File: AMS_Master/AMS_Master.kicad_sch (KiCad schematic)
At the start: 55 parts, among them IC1 LTM2884CY#PBF, IC2 LTC4411ES5#TRMPBF, IC3 ISO1042DWVR, J1 Conn_01x04_Pin, J2 Conn_01x04_Pin, J3 USB_B, J4 Conn_01x14_Pin, U1 LD1117S50TR_SOT223, U2 ADuM1250, U3 MCP2515-xSO, U4 ATmega328P-A, U5 FT232RL, Y1 Crystal, Y2 CSTCE16M0V53-R0

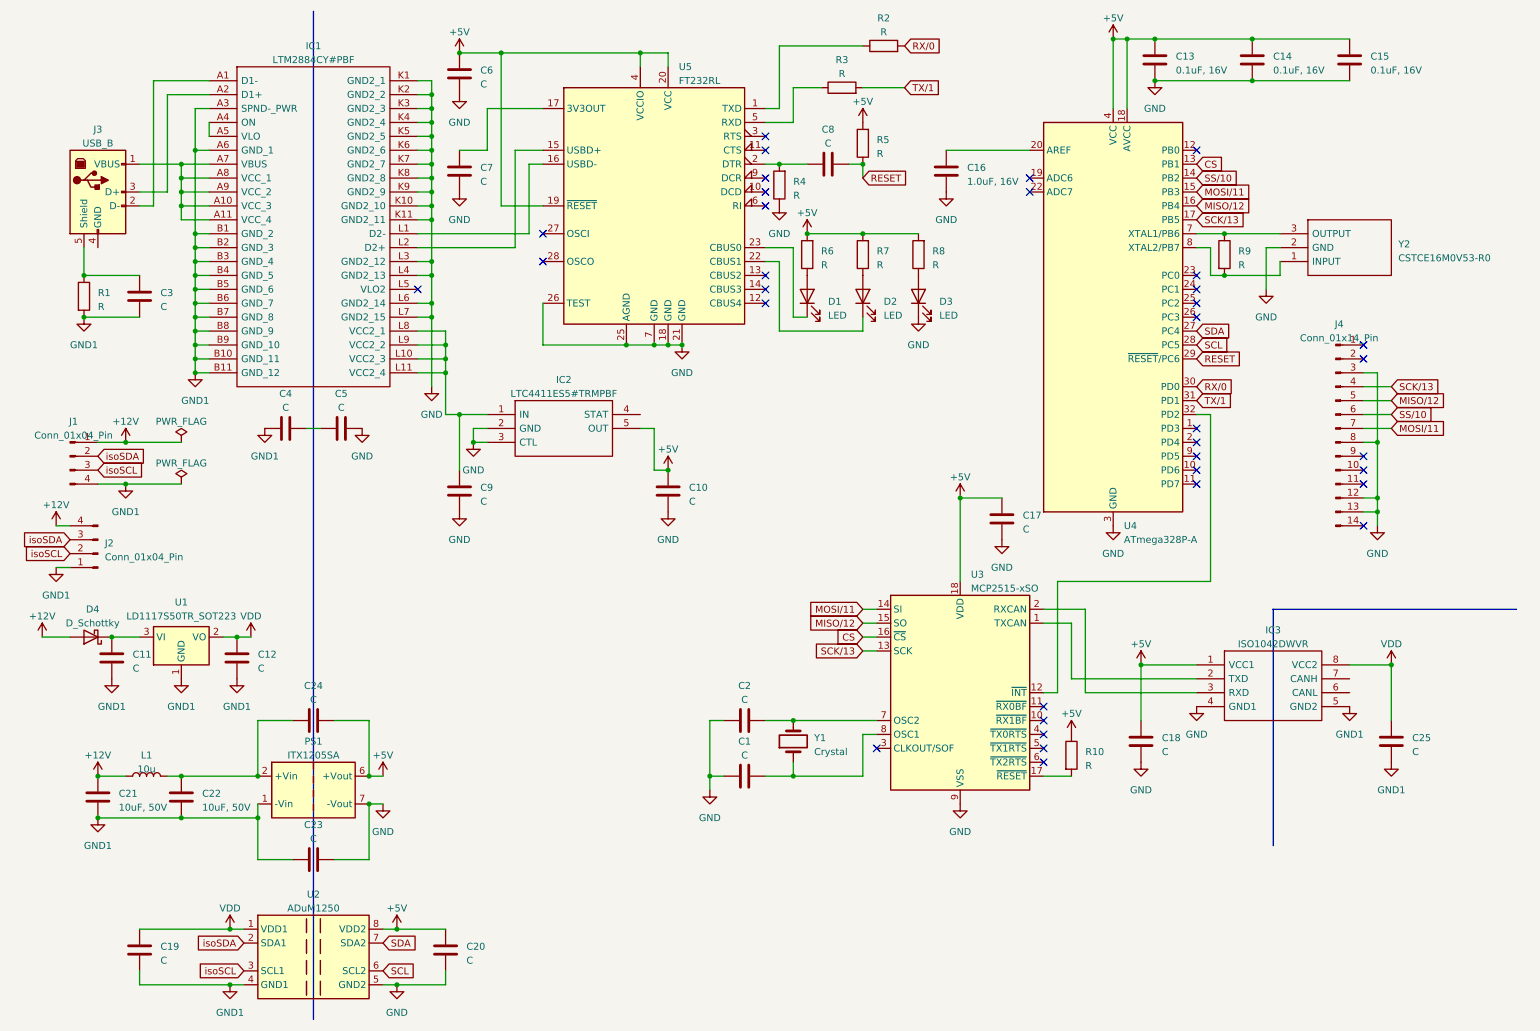
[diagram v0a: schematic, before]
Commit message: AMS_Master回路図更新
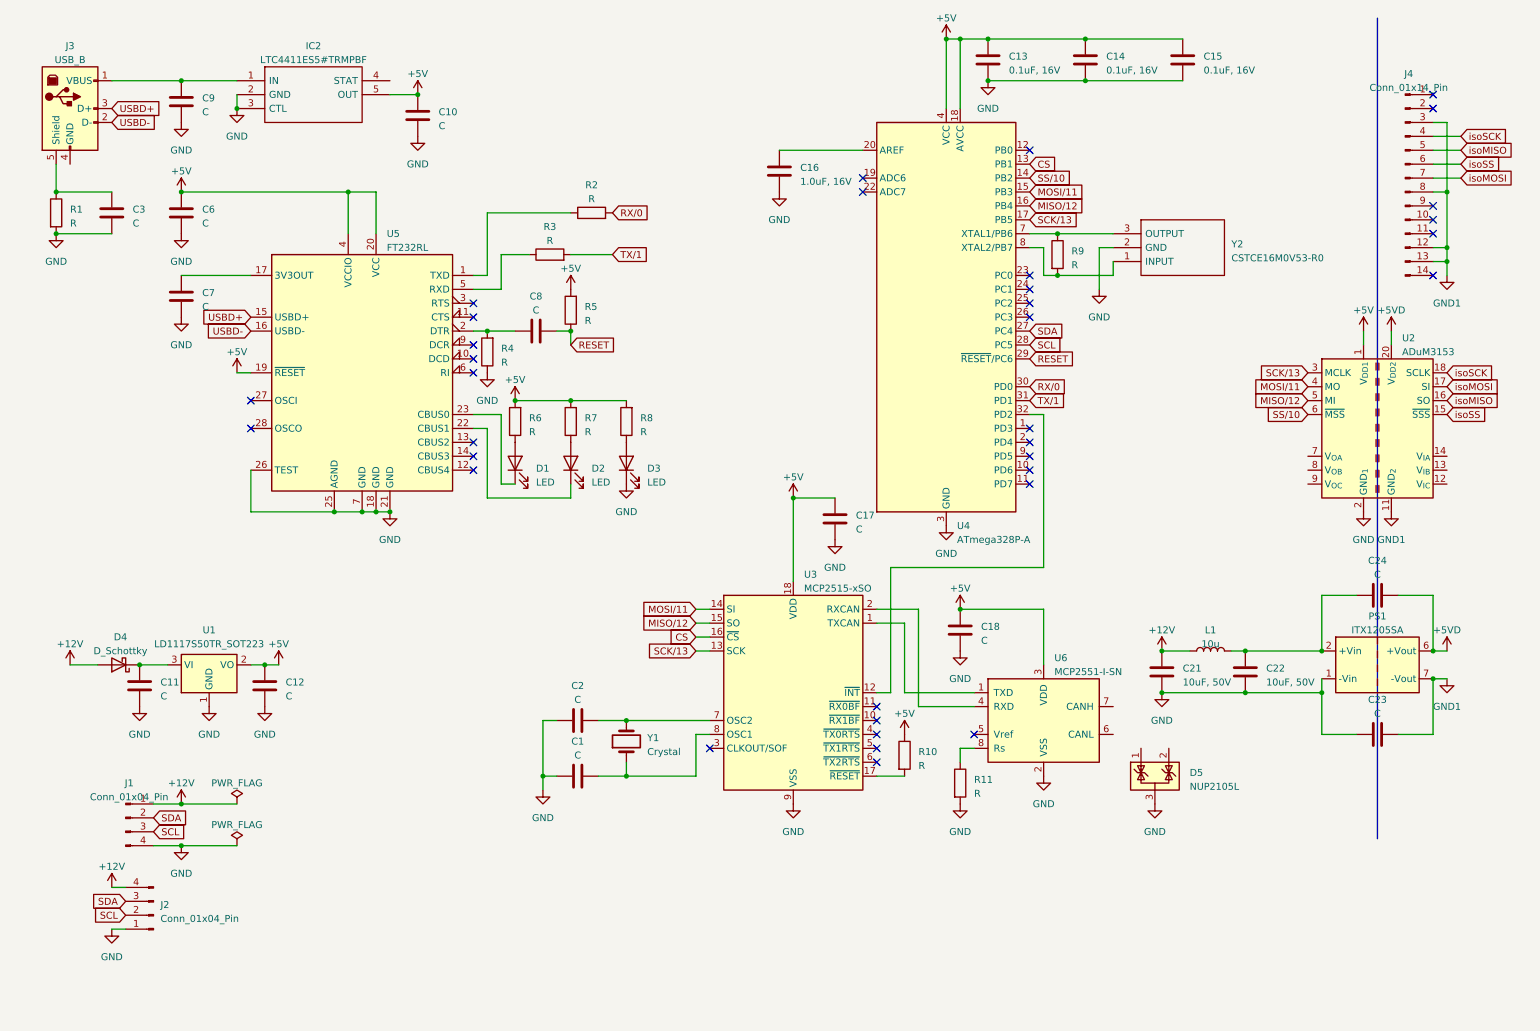
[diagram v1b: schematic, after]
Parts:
- removed C19, C20, C25, C4, C5: C, symbol Device:C
- removed IC1: LTM2884CY#PBF, BGA44C127P11X11_1500X1500X522, symbol SamacSys_Parts:LTM2884CY#PBF
- removed IC3: ISO1042DWVR, SOIC127P1150X280-8N, symbol SamacSys_Parts:ISO1042DWVR
- removed U2: ADuM1250, Package_SO:SOIC-8_3.9x4.9mm_P1.27mm, symbol Isolator:ADuM1250
- added D5: NUP2105L, Package_TO_SOT_SMD:SOT-23, symbol Power_Protection:NUP2105L
- added R11: R, symbol Device:R
- added U2: ADuM3153, Package_SO:SSOP-20_5.3x7.2mm_P0.65mm, symbol Isolator:ADuM3153
- added U6: MCP2551-I-SN, Package_SO:SOIC-8_3.9x4.9mm_P1.27mm, symbol Interface_CAN_LIN:MCP2551-I-SN
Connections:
- net VDD is gone; now on net +5V: C12.1, U1.2 (VO)
- net isoSCL is gone; now on net SCL: J1.3 (Pin_3), J2.2 (Pin_2)
- net isoSDA is gone; now on net SDA: J1.2 (Pin_2), J2.3 (Pin_3)
- net +5V: now also U2.1 (V_{DD1}), U6.3 (VDD); no longer C24.2, PS1.6 (+Vout)
- net GND: now also C11.2, C12.2, C21.2, C22.2, C23.1, C3.2, J1.4 (Pin_4), J2.1 (Pin_1), PS1.1 (-Vin), R1.2, U1.1 (GND), D5.3 (A), R11.2, U2.10 (GND_{1}), U2.2 (GND_{1}), U6.2 (VSS); no longer C23.2, J4.12 (Pin_12), J4.13 (Pin_13), J4.3 (Pin_3), J4.8 (Pin_8), PS1.7 (-Vout)
- net GND1: now also C23.2, J4.12 (Pin_12), J4.13 (Pin_13), J4.3 (Pin_3), J4.8 (Pin_8), PS1.7 (-Vout), U2.11 (GND_{2}), U2.19 (GND_{2}); no longer C11.2, C12.2, C21.2, C22.2, C23.1, C3.2, J1.4 (Pin_4), J2.1 (Pin_1), PS1.1 (-Vin), R1.2, U1.1 (GND)
- net MISO/12: now also U2.5 (MI); no longer J4.5 (Pin_5)
- net MOSI/11: now also U2.4 (MO); no longer J4.7 (Pin_7)
- net SCK/13: now also U2.3 (MCLK); no longer J4.4 (Pin_4)
- net SS/10: now also U2.6 (~{MSS}); no longer J4.6 (Pin_6)
- net at U3.1 (TXCAN): now also U6.1 (TXD)
- net at U3.2 (RXCAN): now also U6.4 (RXD)
- net USBD-: now reaches J3.2 (D-)
- net USBD-: now also U5.16 (USBD-)
- net at J3.1 (VBUS): now also C9.1, IC2.1 (IN)
- net USBD+: now reaches J3.3 (D+)
- net USBD+: now also U5.15 (USBD+)
- new net: R11.1, U6.8 (Rs)
- new net +5VD: C24.2, PS1.6 (+Vout), U2.20 (V_{DD2})
- new net isoMISO: J4.5 (Pin_5), U2.16 (SO)
- new net isoMOSI: J4.7 (Pin_7), U2.17 (SI)
- new net isoSCK: J4.4 (Pin_4), U2.18 (SCLK)
- new net isoSS: J4.6 (Pin_6), U2.15 (~{SSS})
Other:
- moved on the sheet: C1, C10, C11, C12, C13, C14, C15, C16, C17, C18, C2, C21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

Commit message: 回路図更新
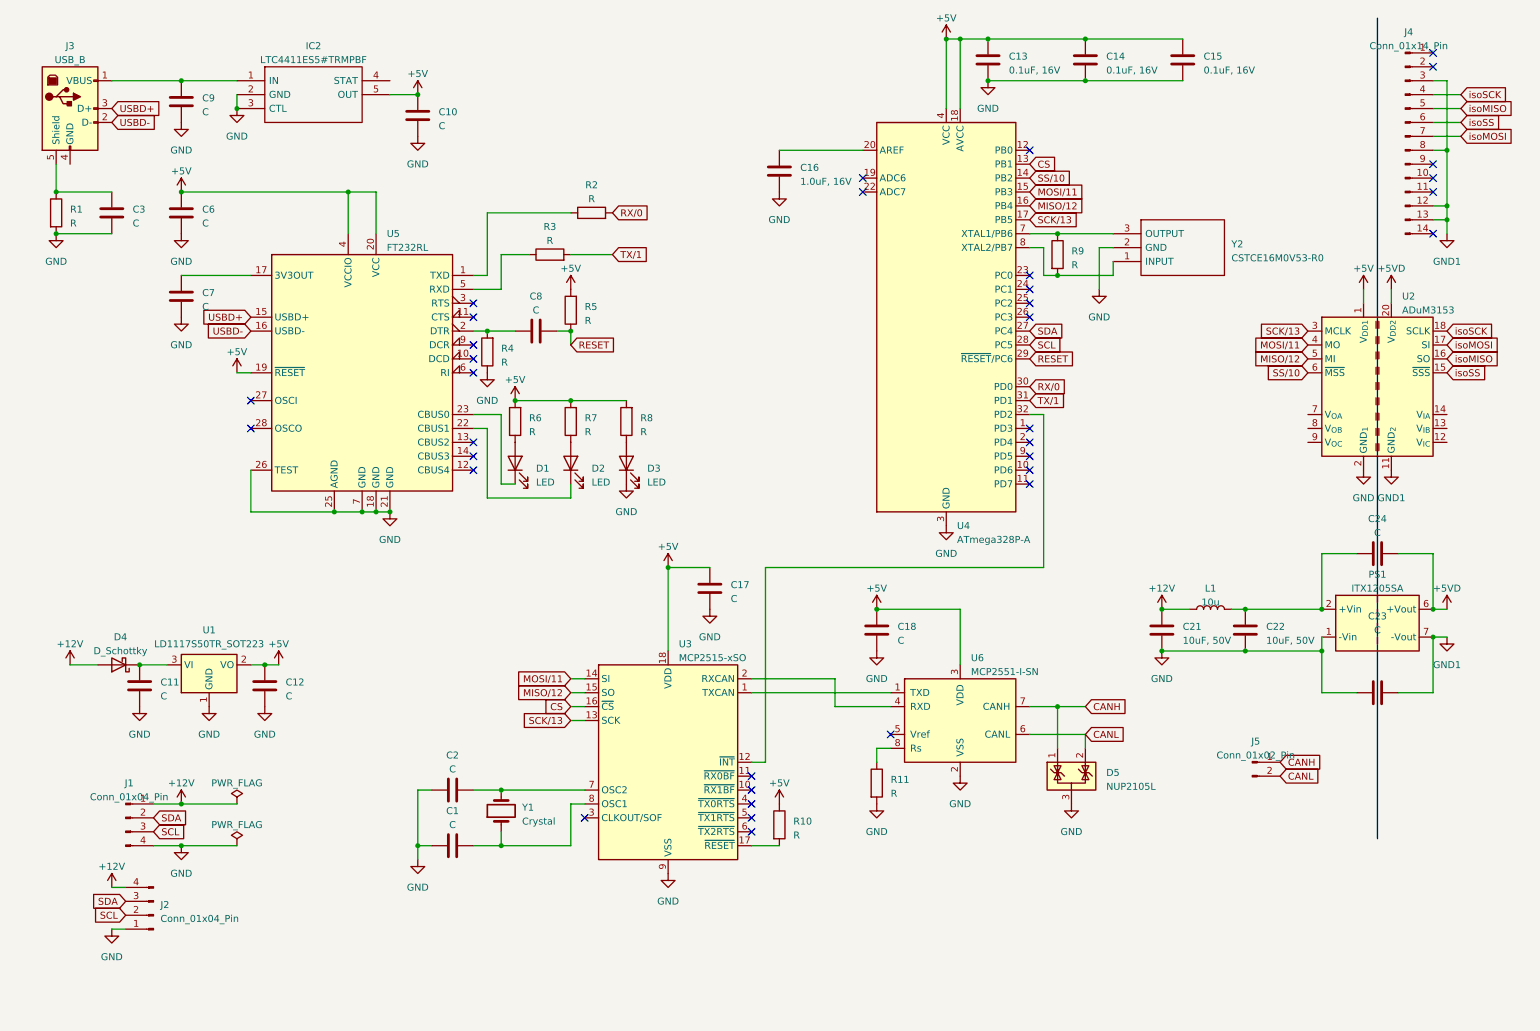
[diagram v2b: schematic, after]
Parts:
- added J5: Conn_01x02_Pin, symbol Connector:Conn_01x02_Pin
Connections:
- net CANL: now reaches U6.6 (CANL)
- net CANL: now also D5.2 (K), J5.2 (Pin_2)
- net CANH: now reaches U6.7 (CANH)
- net CANH: now also D5.1 (K), J5.1 (Pin_1)
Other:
- moved on the sheet: C1, C17, C18, C2, C21, C22, C23, C24, D5, J4, L1, PS1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

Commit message: 回路図更新
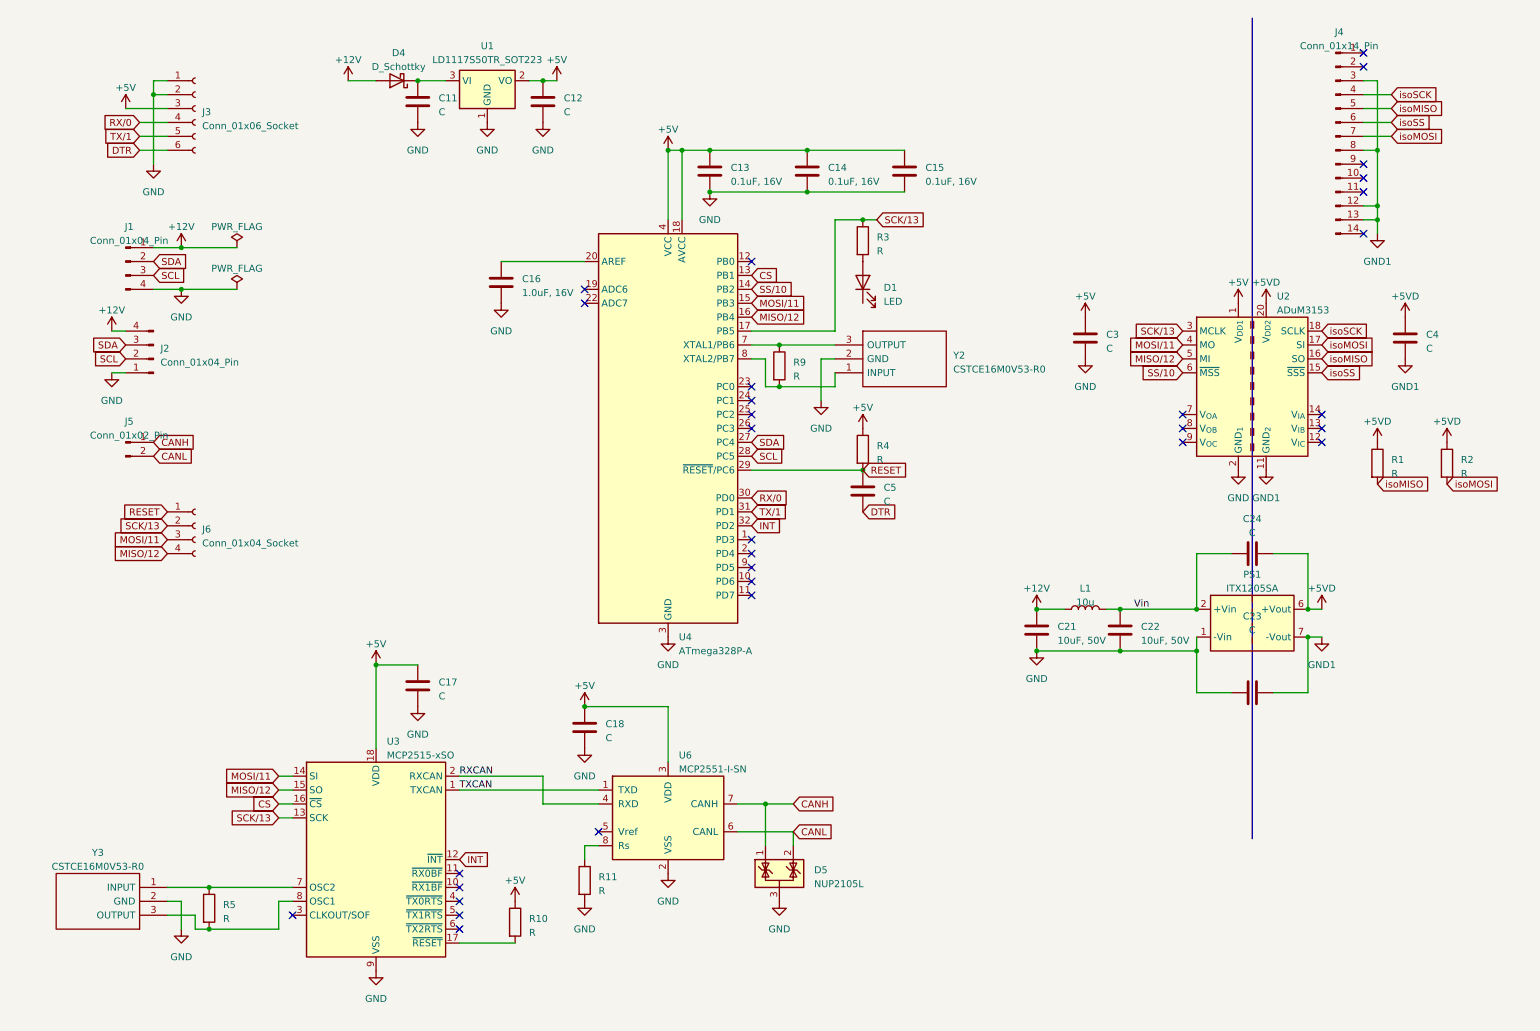
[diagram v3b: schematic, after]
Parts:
- removed C1, C10, C2, C6, C7, C8, C9: C, symbol Device:C
- removed D2, D3: LED, symbol Device:LED
- removed IC2: LTC4411ES5#TRMPBF, SOT95P280X100-5N, symbol SamacSys_Parts:LTC4411ES5#TRMPBF
- removed J3: USB_B, symbol Connector:USB_B
- removed R6, R7, R8: R, symbol Device:R
- removed U5: FT232RL, Package_SO:SSOP-28_5.3x10.2mm_P0.65mm, symbol Interface_USB:FT232RL
- removed Y1: Crystal, symbol Device:Crystal
- added C4, C5: C, symbol Device:C
- added J3: Conn_01x06_Socket, symbol Connector:Conn_01x06_Socket
- added J6: Conn_01x04_Socket, symbol Connector:Conn_01x04_Socket
- added Y3: CSTCE16M0V53-R0, CSTCE16M0V53R0, symbol SamacSys_Parts:CSTCE16M0V53-R0
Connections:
- net +5V: now also C3.1, R4.1, J3.3 (Pin_3); no longer R5.2
- net +5VD: now also R1.1, R2.1, C4.1
- net GND: now also J3.1 (Pin_1), J3.2 (Pin_2), Y3.2 (GND); no longer R1.2, R4.1
- net GND1: now also C4.2
- net MISO/12: now also J6.4 (Pin_4)
- net MOSI/11: now also J6.3 (Pin_3)
- net RESET: now also R4.2, C5.1, J6.1 (Pin_1); no longer R5.1
- net RX/0: now also J3.4 (Pin_4); no longer R2.2
- net SCK/13: now also R3.1, J6.2 (Pin_2)
- net TX/1: now also J3.5 (Pin_5); no longer R3.2
- net isoMISO: now also R1.2
- net isoMOSI: now also R2.2
- net at U3.8 (OSC1): now also R5.2, Y3.3 (OUTPUT)
- net at U3.7 (OSC2): now also R5.1, Y3.1 (INPUT)
- net Vin: now reaches C22.1, C24.1, L1.2, PS1.2 (+Vin)
- net TXCAN: now reaches U3.1 (TXCAN), U6.1 (TXD)
- net INT: now reaches U3.12 (~{INT}), U4.32 (PD2)
- net RXCAN: now reaches U3.2 (RXCAN), U6.4 (RXD)
- net at D1.2 (A): now also R3.2
- new net DTR: C5.2, J3.6 (Pin_6)
- no-connect marks 35 -> 31
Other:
- moved on the sheet: C11, C12, C13, C14, C15, C16, C17, C18, C21, C22, C23, C24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
